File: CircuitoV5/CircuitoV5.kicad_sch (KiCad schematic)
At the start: 18 parts, among them J1 Conn_01x05, J2 Screw_Terminal_01x02, J3 Screw_Terminal_01x02, U1 LM324, U2 LM358

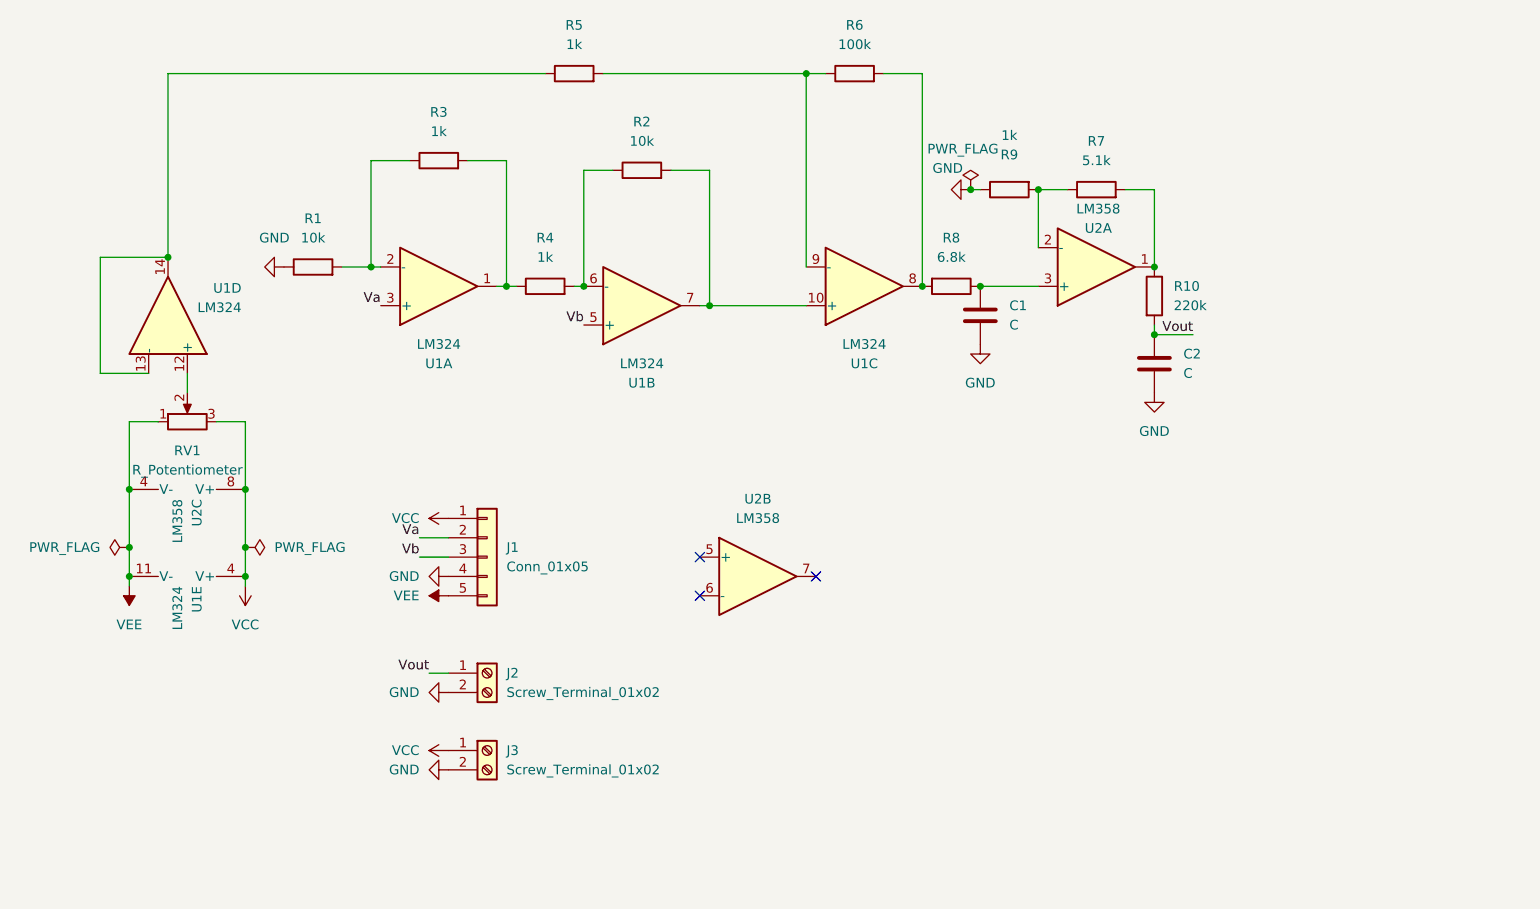
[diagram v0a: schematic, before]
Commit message: Routed and done
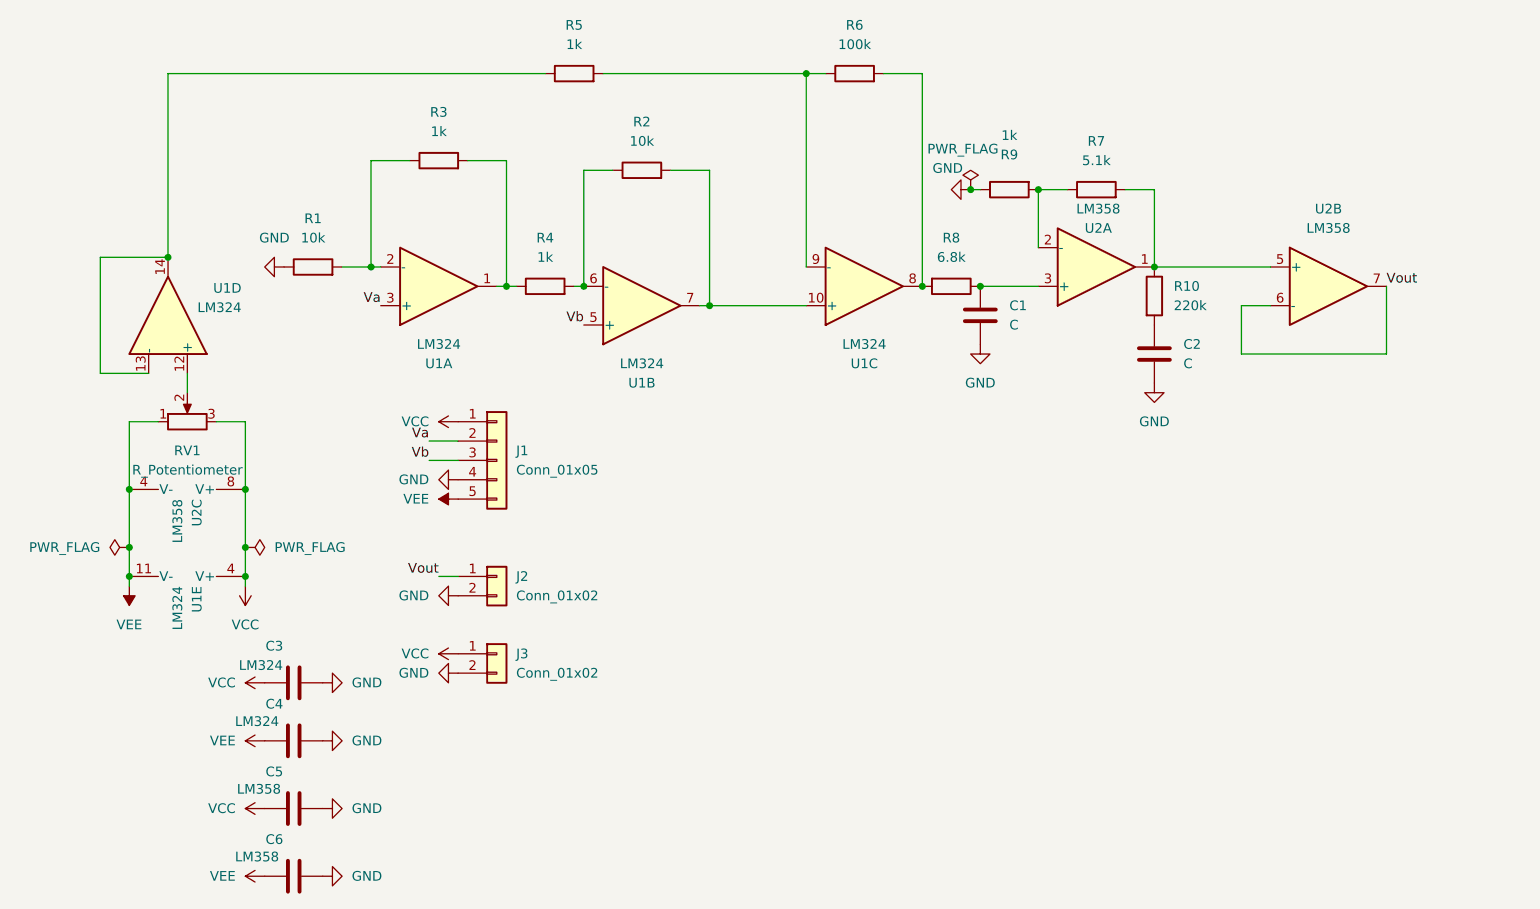
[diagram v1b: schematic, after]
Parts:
- removed J2, J3: Screw_Terminal_01x02, TerminalBlock_Phoenix:TerminalBlock_Phoenix_MKDS-1,5-2-5.08_1x02_P5.08mm_Horizontal, symbol Connector:Screw_Terminal_01x02
- added C3, C4: LM324, Capacitor_THT:C_Disc_D5.0mm_W2.5mm_P2.50mm, symbol Device:C
- added C5, C6: LM358, Capacitor_THT:C_Disc_D5.0mm_W2.5mm_P2.50mm, symbol Device:C
- added J2, J3: Conn_01x02, Connector_PinSocket_2.54mm:PinSocket_1x02_P2.54mm_Vertical, symbol Connector_Generic:Conn_01x02
- R1, R2, R7: footprint Resistor_SMD:R_0402_1005Metric -> Resistor_THT:R_Axial_DIN0207_L6.3mm_D2.5mm_P10.16mm_Horizontal
- R10, R8: footprint Resistor_SMD:R_0201_0603Metric -> Resistor_THT:R_Axial_DIN0207_L6.3mm_D2.5mm_P10.16mm_Horizontal
- R3, R4, R5, R6, R9: footprint Resistor_SMD:R_0603_1608Metric -> Resistor_THT:R_Axial_DIN0207_L6.3mm_D2.5mm_P10.16mm_Horizontal
- U1: footprint easyeda2kicad:PDIP-14_L19.7-W6.6-P2.54-LS8.3-BL -> Package_DIP:DIP-14_W7.62mm
- U2: footprint footprints:DIP794W45P254L959H508Q8 -> Package_DIP:DIP-8_W7.62mm
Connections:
- net GND: now also C3.2, C4.2, C5.2, C6.2, J2.2 (Pin_2), J3.2 (Pin_2)
- net VCC: now also C3.1, C5.1, J3.1 (Pin_1)
- net VEE: now also C4.1, C6.1
- net Vout: now also U2.6 (-), U2.7, J2.1 (Pin_1); no longer C2.1, R10.2
- net at R10.1, R7.2, U2.1: now also U2.5 (+)
- new net: C2.1, R10.2
- no-connect marks 3 -> 0
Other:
- moved on the sheet: C2, J1, U2B

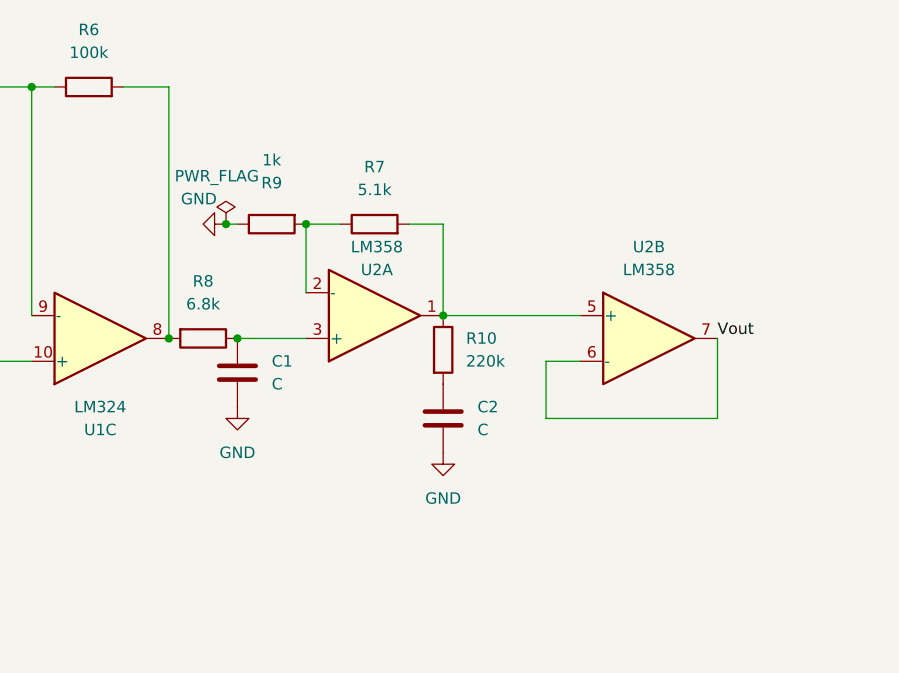
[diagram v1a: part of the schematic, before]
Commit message: Ultimas actualizaciones y correcciones
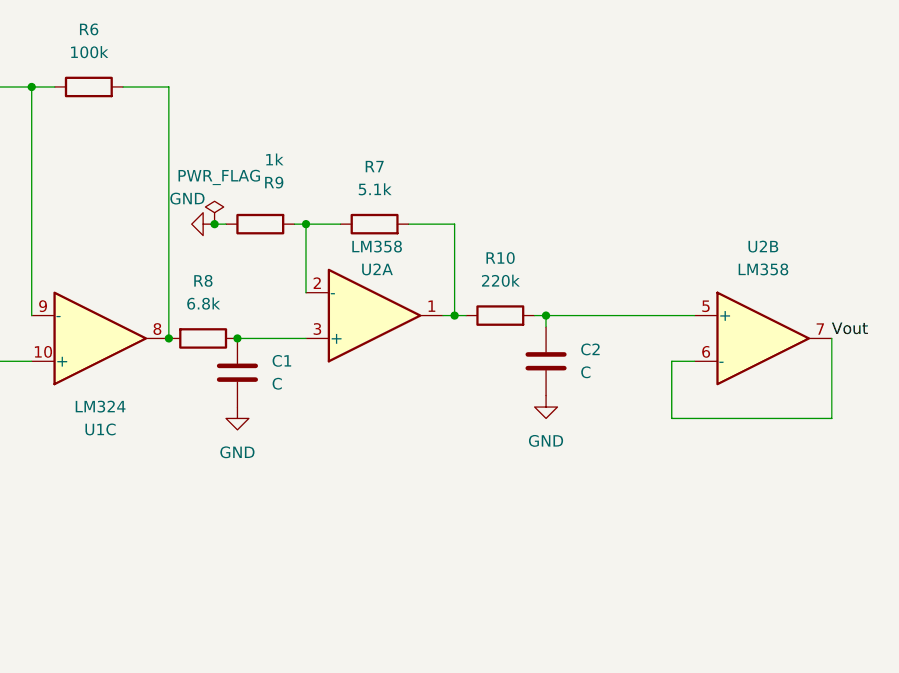
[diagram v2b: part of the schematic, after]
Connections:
- net at R10.1, R7.2, U2.1: no longer U2.5 (+)
- net at C2.1, R10.2: now also U2.5 (+)
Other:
- moved on the sheet: C2, R10, R9, U2B
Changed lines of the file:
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@@
 	(paper "A4")
 	(junction
-		(at 157.48 43.18)
+		(at 156.21 43.18)
 		(diameter 0)
 		(color 0 0 0 0)
@@
 	)
 	(junction
-		(at 46.99 90.17)
+		(at 193.04 53.34)
 		(diameter 0)
 		(color 0 0 0 0)
 	)
 	(junction
-		(at 181.61 53.34)
+		(at 46.99 90.17)
 		(diameter 0)
 		(color 0 0 0 0)
@@
 	)
 	(junction
+		(at 182.88 53.34)
+		(diameter 0)
+		(color 0 0 0 0)
+	)
+	(junction
 		(at 96.52 55.88)
 		(diameter 0)
@@
 	(wire
 		(pts
-			(xy 181.61 53.34) (xy 196.85 53.34)
+			(xy 156.21 43.18) (xy 157.48 43.18)
 		)
 		(stroke
@@
 	(wire
 		(pts
-			(xy 157.48 43.18) (xy 158.75 43.18)
+			(xy 62.23 95.25) (xy 62.23 93.98)
 		)
 		(stroke
@@
 	(wire
 		(pts
-			(xy 62.23 95.25) (xy 62.23 93.98)
+			(xy 193.04 53.34) (xy 209.55 53.34)
 		)
 		(stroke
@@
 	(wire
 		(pts
-			(xy 196.85 58.42) (xy 193.04 58.42)
+			(xy 209.55 58.42) (xy 207.01 58.42)
 		)
 		(stroke
@@
 	(wire
 		(pts
-			(xy 181.61 43.18) (xy 181.61 53.34)
+			(xy 182.88 43.18) (xy 182.88 53.34)
+		)
+		(stroke
+			(width 0)
+			(type default)
+		)
+	)
+	(wire
+		(pts
+			(xy 184.15 53.34) (xy 182.88 53.34)
+		)
+		(stroke
+			(width 0)
+			(type default)
+		)
+	)
+	(wire
+		(pts
+			(xy 182.88 53.34) (xy 181.61 53.34)
 		)
 		(stroke
@@
 	(wire
 		(pts
-			(xy 212.09 64.77) (xy 212.09 55.88)
+			(xy 224.79 64.77) (xy 224.79 55.88)
 		)
 		(stroke
@@
 	(wire
 		(pts
+			(xy 165.1 43.18) (xy 166.37 43.18)
+		)
+		(stroke
+			(width 0)
+			(type default)
+		)
+	)
+	(wire
+		(pts
 			(xy 86.36 76.2) (xy 90.17 76.2)
 		)
@@
 	(wire
 		(pts
-			(xy 193.04 64.77) (xy 212.09 64.77)
+			(xy 207.01 64.77) (xy 224.79 64.77)
+		)
+		(stroke
+			(width 0)
+			(type default)
+		)
+	)
+	(wire
+		(pts
+			(xy 193.04 53.34) (xy 193.04 54.61)
 		)
 		(stroke
@@
 	(wire
 		(pts
-			(xy 177.8 43.18) (xy 181.61 43.18)
+			(xy 177.8 43.18) (xy 182.88 43.18)
 		)
 		(stroke
@@
 	(wire
 		(pts
-			(xy 193.04 58.42) (xy 193.04 64.77)
+			(xy 207.01 58.42) (xy 207.01 64.77)
 		)
 		(stroke
@@
 	(wire
 		(pts
+			(xy 191.77 53.34) (xy 193.04 53.34)
+		)
+		(stroke
+			(width 0)
+			(type default)
+		)
+	)
+	(wire
+		(pts
 			(xy 106.68 55.88) (xy 106.68 40.64)
 		)
@@
 	)
 	(label "Vout"
-		(at 212.09 55.88 0)
+		(at 224.79 55.88 0)
 		(effects
 			(font
@@
 	(symbol
 		(lib_id "Device:R")
-		(at 162.56 43.18 90)
+		(at 161.29 43.18 90)
 		(mirror x)
 		(unit 1)
@@
 		(dnp no)
 		(property "Reference" "R9"
-			(at 162.56 38.608 90)
+			(at 162.814 38.608 90)
 			(show_name no)
 			(do_not_autoplace no)
@@
 		)
 		(property "Value" "1k"
-			(at 162.56 36.068 90)
+			(at 162.814 36.068 90)
 			(show_name no)
 			(do_not_autoplace no)
@@
 		)
 		(property "Footprint" "Resistor_THT:R_Axial_DIN0207_L6.3mm_D2.5mm_P10.16mm_Horizontal"
-			(at 162.56 41.402 90)
+			(at 161.29 41.402 90)
 			(hide yes)
 			(show_name no)
@@
 		)
 		(property "Datasheet" ""
-			(at 162.56 43.18 0)
+			(at 161.29 43.18 0)
 			(hide yes)
 			(show_name no)
@@
 		)
 		(property "Description" "Resistor"
-			(at 162.56 43.18 0)
+			(at 161.29 43.18 0)
 			(hide yes)
 			(show_name no)
@@
 		)
 		(property "LCSC_Id" "C21190"
-			(at 162.56 43.18 0)
+			(at 161.29 43.18 0)
 			(hide yes)
 			(show_name no)
@@
 	(symbol
 		(lib_id "power:PWR_FLAG")
-		(at 157.48 43.18 0)
+		(at 156.21 43.18 0)
 		(unit 1)
 		(body_style 1)
@@
 		(dnp no)
 		(property "Reference" "#FLG03"
-			(at 157.48 41.275 0)
+			(at 156.21 41.275 0)
 			(hide yes)
 			(show_name no)
@@
 		)
 		(property "Value" "PWR_FLAG"
-			(at 156.464 37.846 0)
+			(at 156.718 37.846 0)
 			(show_name no)
 			(do_not_autoplace no)
@@
 		)
 		(property "Footprint" ""
-			(at 157.48 43.18 0)
+			(at 156.21 43.18 0)
 			(hide yes)
 			(show_name no)
@@
 		)
 		(property "Datasheet" ""
-			(at 157.48 43.18 0)
+			(at 156.21 43.18 0)
 			(hide yes)
 			(show_name no)
@@
 		)
 		(property "Description" "Special symbol for telling ERC where power comes from"
-			(at 157.48 43.18 0)
+			(at 156.21 43.18 0)
 			(hide yes)
 			(show_name no)
@@
 	(symbol
 		(lib_id "Device:R")
-		(at 181.61 57.15 0)
+		(at 187.96 53.34 90)
 		(unit 1)
 		(body_style 1)
@@
 		(fields_autoplaced yes)
 		(property "Reference" "R10"
-			(at 184.15 55.8799 0)
+			(at 187.96 46.99 90)
 			(show_name no)
 			(do_not_autoplace no)
@@
 					(size 1.27 1.27)
 				)
-				(justify left)
 			)
 		)
 		(property "Value" "220k"
-			(at 184.15 58.4199 0)
+			(at 187.96 49.53 90)
 			(show_name no)
 			(do_not_autoplace no)
@@
 					(size 1.27 1.27)
 				)
-				(justify left)
 			)
 		)
 		(property "Footprint" "Resistor_THT:R_Axial_DIN0207_L6.3mm_D2.5mm_P10.16mm_Horizontal"
-			(at 179.832 57.15 90)
+			(at 187.96 55.118 90)
 			(hide yes)
 			(show_name no)
@@
 		)
 		(property "Datasheet" ""
-			(at 181.61 57.15 0)
+			(at 187.96 53.34 0)
 			(hide yes)
 			(show_name no)
@@
 		)
 		(property "Description" "Resistor"
-			(at 181.61 57.15 0)
+			(at 187.96 53.34 0)
 			(hide yes)
 			(show_name no)
@@
 		)
 		(property "LCSC_Id" "C2907013"
-			(at 181.61 57.15 0)
+			(at 187.96 53.34 0)
 			(hide yes)
 			(show_name no)
@@
 	(symbol
 		(lib_id "power:GND")
-		(at 181.61 68.58 0)
+		(at 193.04 62.23 0)
 		(unit 1)
 		(body_style 1)
@@
 		(fields_autoplaced yes)
 		(property "Reference" "#PWR04"
-			(at 181.61 74.93 0)
+			(at 193.04 68.58 0)
 			(hide yes)
 			(show_name no)
@@
 		)
 		(property "Value" "GND"
-			(at 181.61 73.66 0)
+			(at 193.04 67.31 0)
 			(show_name no)
 			(do_not_autoplace no)
@@
 		)
 		(property "Footprint" ""
-			(at 181.61 68.58 0)
+			(at 193.04 62.23 0)
 			(hide yes)
 			(show_name no)
@@
 		)
 		(property "Datasheet" ""
-			(at 181.61 68.58 0)
+			(at 193.04 62.23 0)
 			(hide yes)
 			(show_name no)
@@
 		)
 		(property "Description" "Power symbol creates a global label with name \"GND\" , ground"
-			(at 181.61 68.58 0)
+			(at 193.04 62.23 0)
 			(hide yes)
 			(show_name no)
@@
 	(symbol
 		(lib_id "Device:C")
-		(at 181.61 64.77 0)
+		(at 193.04 58.42 0)
 		(unit 1)
 		(body_style 1)
@@
 		(dnp no)
 		(property "Reference" "C2"
-			(at 185.42 63.4999 0)
+			(at 196.85 57.1499 0)
 			(show_name no)
 			(do_not_autoplace no)
@@
 		)
 		(property "Value" "C"
-			(at 185.42 66.0399 0)
+			(at 196.85 59.6899 0)
 			(show_name no)
 			(do_not_autoplace no)
@@
 		)
 		(property "Footprint" "footprints:C_Rect_L9.5mm_W4.5mm_P5.00mm_MKT"
-			(at 182.5752 68.58 0)
+			(at 194.0052 62.23 0)
 			(hide yes)
 			(show_name no)
@@
 		)
 		(property "Datasheet" ""
-			(at 181.61 64.77 0)
+			(at 193.04 58.42 0)
 			(hide yes)
 			(show_name no)
@@
 		)
 		(property "Description" "Unpolarized capacitor"
-			(at 181.61 64.77 0)
+			(at 193.04 58.42 0)
 			(hide yes)
 			(show_name no)
@@
 	(symbol
 		(lib_id "power:GND")
-		(at 157.48 43.18 270)
+		(at 156.21 43.18 270)
 		(unit 1)
 		(body_style 1)
@@
 		(dnp no)
 		(property "Reference" "#PWR01"
-			(at 151.13 43.18 0)
+			(at 149.86 43.18 0)
 			(hide yes)
 			(show_name no)
@@
 		)
 		(property "Value" "GND"
-			(at 156.464 40.386 90)
+			(at 155.194 40.386 90)
 			(show_name no)
 			(do_not_autoplace no)
@@
 		)
 		(property "Footprint" ""
-			(at 157.48 43.18 0)
+			(at 156.21 43.18 0)
 			(hide yes)
 			(show_name no)
@@
 		)
 		(property "Datasheet" ""
-			(at 157.48 43.18 0)
+			(at 156.21 43.18 0)
 			(hide yes)
 			(show_name no)
@@
 		)
 		(property "Description" "Power symbol creates a global label with name \"GND\" , ground"
-			(at 157.48 43.18 0)
+			(at 156.21 43.18 0)
 			(hide yes)
 			(show_name no)
@@
 	(symbol
 		(lib_id "Amplifier_Operational:LM358")
-		(at 204.47 55.88 0)
+		(at 217.17 55.88 0)
 		(unit 2)
 		(body_style 1)
@@
 		(fields_autoplaced yes)
 		(property "Reference" "U2"
-			(at 204.47 45.72 0)
+			(at 217.17 45.72 0)
 			(show_name no)
 			(do_not_autoplace no)
@@
 		)
 		(property "Value" "LM358"
-			(at 204.47 48.26 0)
+			(at 217.17 48.26 0)
 			(show_name no)
 			(do_not_autoplace no)
@@
 		)
 		(property "Footprint" "Package_DIP:DIP-8_W7.62mm"
-			(at 204.47 55.88 0)
+			(at 217.17 55.88 0)
 			(hide yes)
 			(show_name no)
@@
 		)
 		(property "Datasheet" "http://www.ti.com/lit/ds/symlink/lm2904-n.pdf"
-			(at 204.47 55.88 0)
+			(at 217.17 55.88 0)
 			(hide yes)
 			(show_name no)
@@
 		)
 		(property "Description" "Low-Power, Dual Operational Amplifiers, DIP-8/SOIC-8/TO-99-8"
-			(at 204.47 55.88 0)
+			(at 217.17 55.88 0)
 			(hide yes)
 			(show_name no)
@@
 		)
 		(property "LCSC_Id" "C5213"
-			(at 204.47 55.88 0)
+			(at 217.17 55.88 0)
 			(hide yes)
 			(show_name no)
